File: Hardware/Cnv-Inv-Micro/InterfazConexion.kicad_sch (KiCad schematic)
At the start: 14 parts, among them J2 Screw_Terminal_01x07, J3 Screw_Terminal_01x03

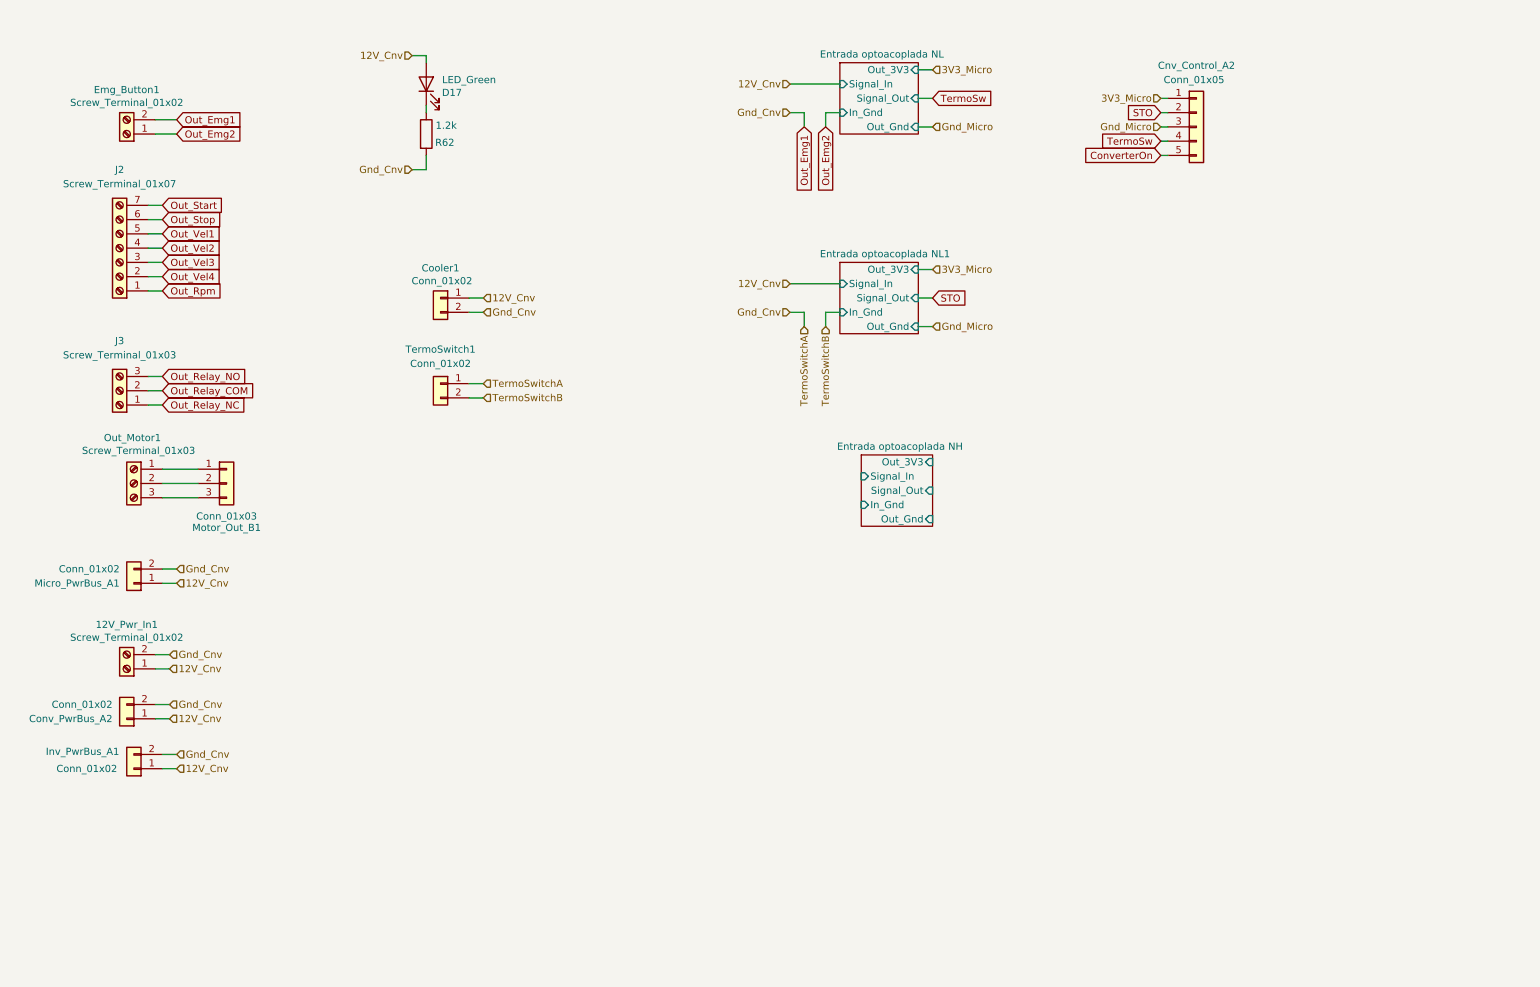
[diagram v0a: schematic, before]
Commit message: Normalizacion placa micros
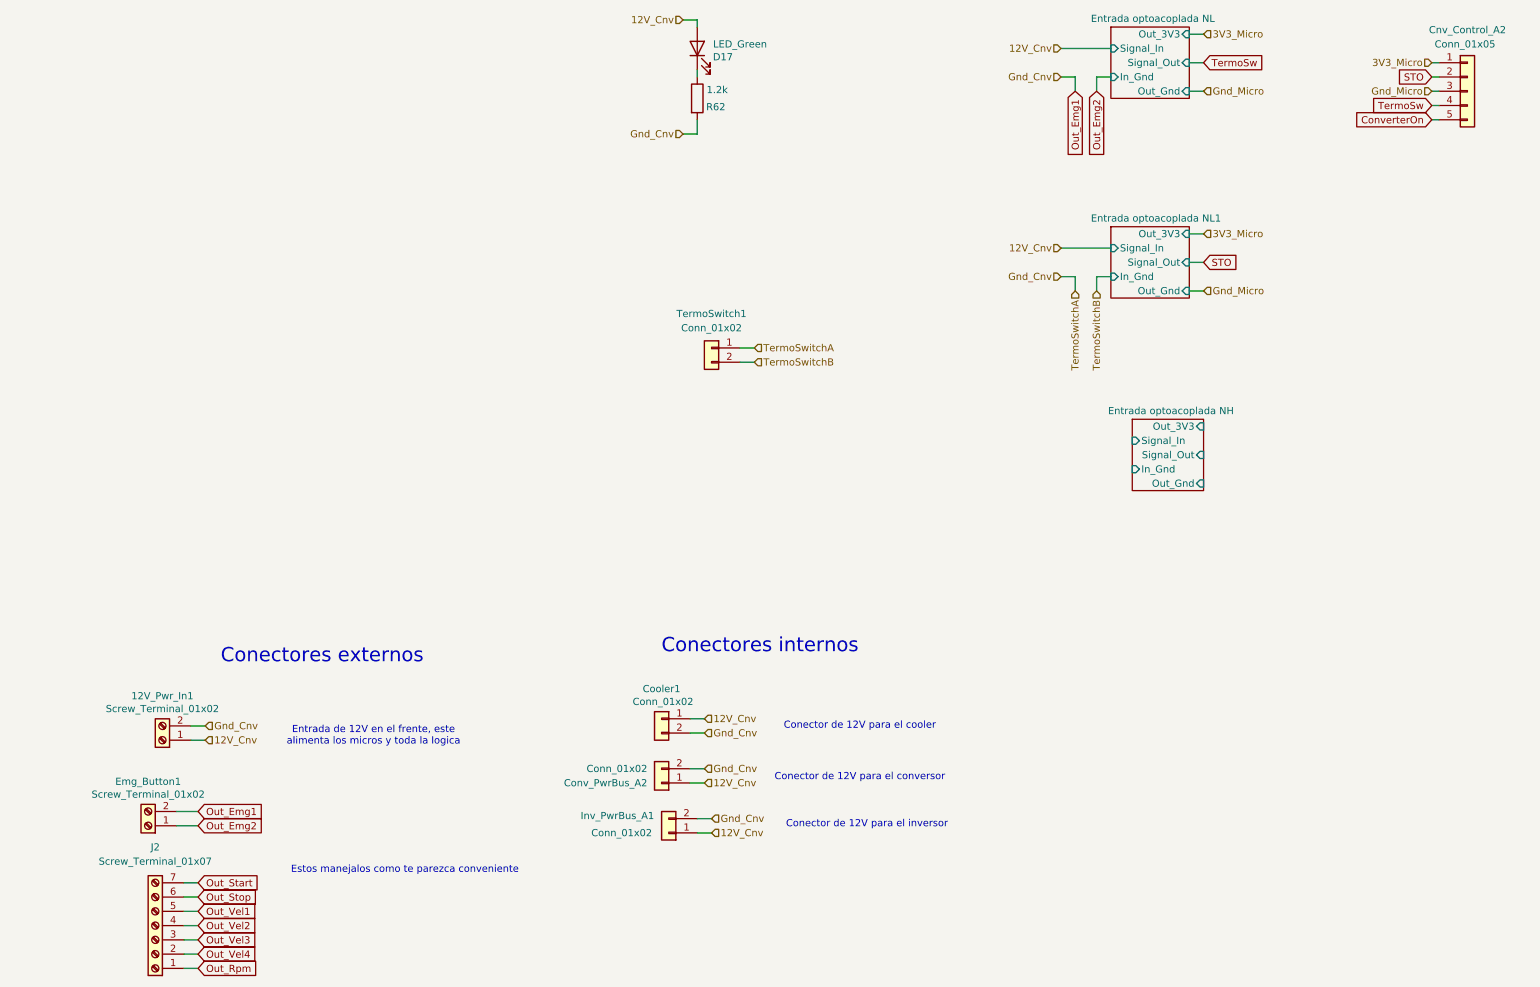
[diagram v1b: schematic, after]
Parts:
- removed J3: Screw_Terminal_01x03, TerminalBlock_Phoenix:TerminalBlock_Phoenix_MKDS-1,5-3-5.08_1x03_P5.08mm_Horizontal, symbol Connector:Screw_Terminal_01x03
- removed Micro_PwrBus_A1: Conn_01x02, Connector_Phoenix_MSTB:PhoenixContact_MSTBVA_2,5_2-G-5,08_1x02_P5.08mm_Vertical, symbol Connector_Generic:Conn_01x02
- removed Motor_Out_B1: Conn_01x03, Connector_Phoenix_MC_HighVoltage:PhoenixContact_MCV_1,5_3-G-5.08_1x03_P5.08mm_Vertical, symbol Connector_Generic:Conn_01x03
- removed Out_Motor1: Screw_Terminal_01x03, TerminalBlock_MetzConnect:TerminalBlock_MetzConnect_Type703_RT10N03HGLU_1x03_P9.52mm_Horizontal, symbol Connector:Screw_Terminal_01x03
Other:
- note added: "Conector de 12V para el conversor"
- note added: "Conector de 12V para el cooler"
- note added: "Conector de 12V para el inversor"
- note added: "Conectores externos"
- note added: "Conectores internos"
- note added: "Entrada de 12V en el frente, este alimenta los micros y toda la logica"
- note added: "Estos manejalos como te parezca conveniente"
- moved on the sheet: 12V_Pwr_In1, Cnv_Control_A2, Conv_PwrBus_A2, Cooler1, D17, Emg_Button1, Inv_PwrBus_A1, J2, R62, TermoSwitch1
